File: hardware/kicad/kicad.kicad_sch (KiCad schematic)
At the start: 4 parts, among them U1 RP2040

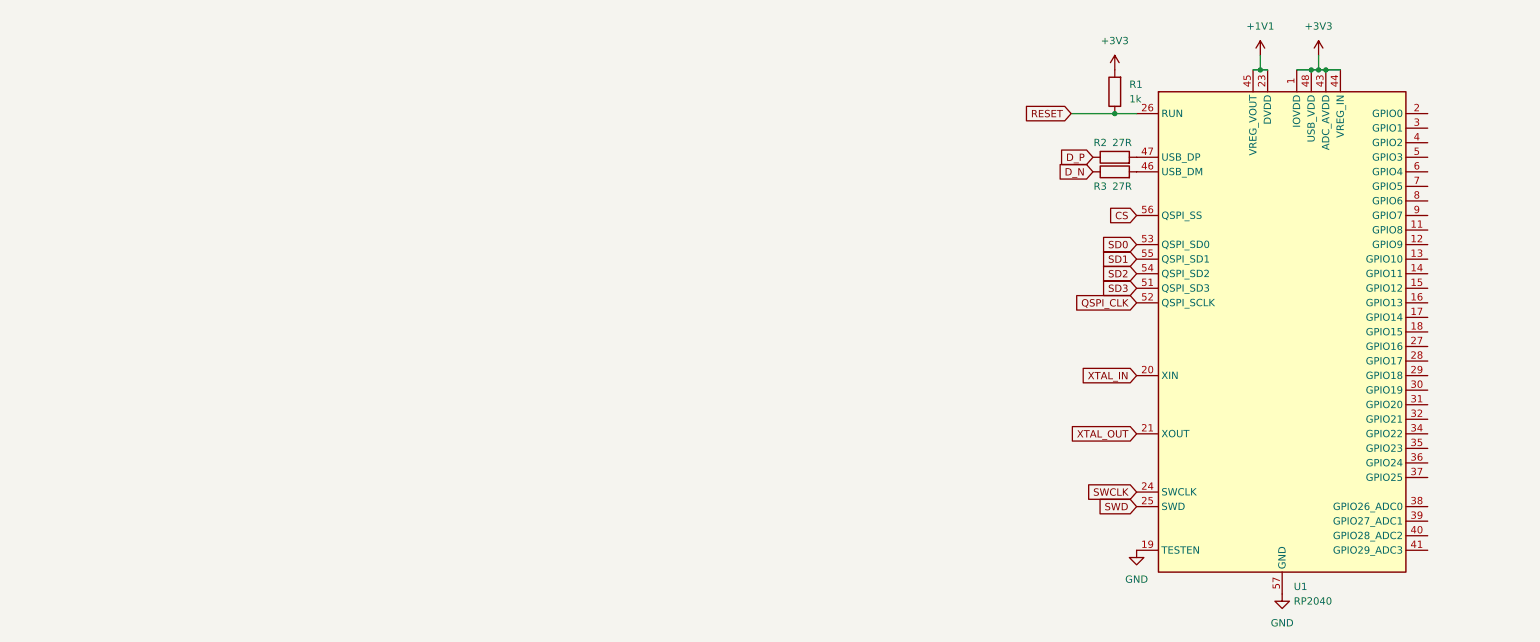
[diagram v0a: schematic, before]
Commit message: [30-8] update progress
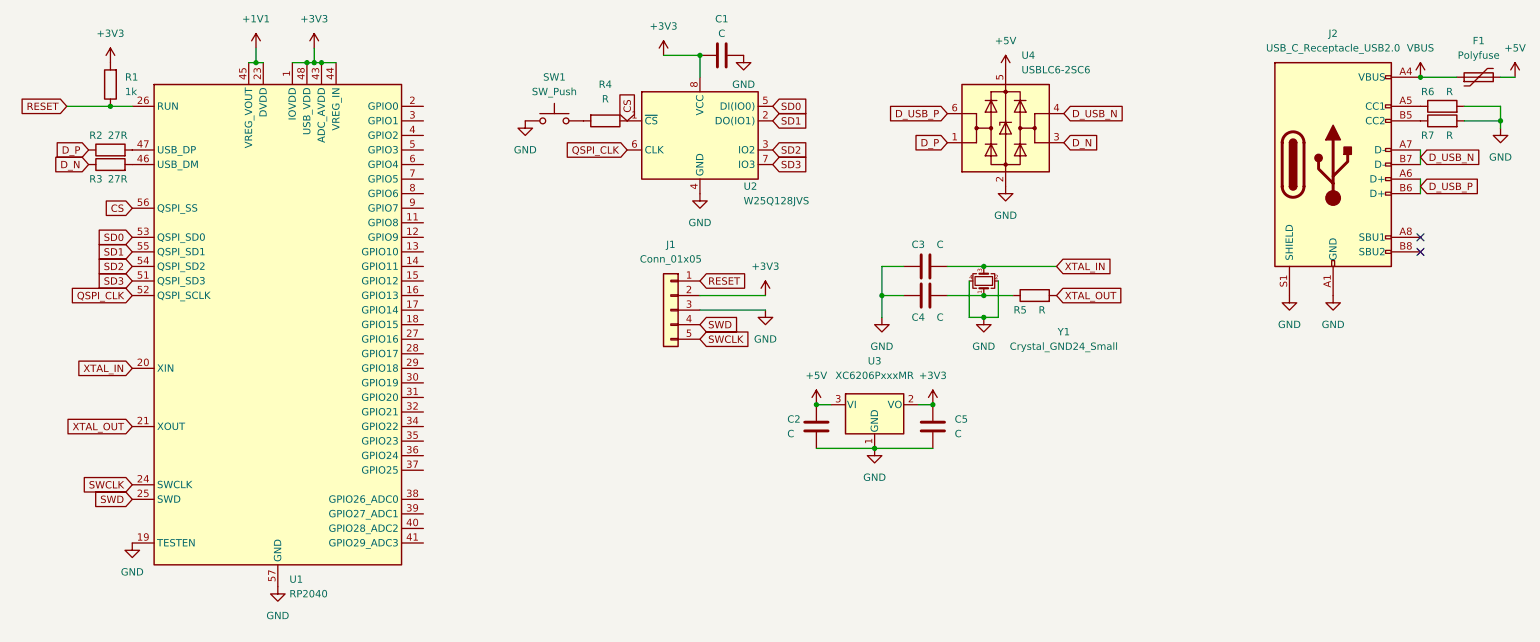
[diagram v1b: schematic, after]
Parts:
- added C1, C2, C3, C4, C5: C, Capacitor_SMD:C_0603_1608Metric_Pad1.08x0.95mm_HandSolder, symbol Device:C
- added F1: Polyfuse, Fuse:Fuse_0603_1608Metric_Pad1.05x0.95mm_HandSolder, symbol Device:Polyfuse
- added J1: Conn_01x05, Connector_PinHeader_2.54mm:PinHeader_1x05_P2.54mm_Vertical, symbol Connector_Generic:Conn_01x05
- added J2: USB_C_Receptacle_USB2.0, Connector_USB:USB_C_Receptacle_HRO_TYPE-C-31-M-12, symbol Connector:USB_C_Receptacle_USB2.0
- added R4, R5, R6, R7: R, Resistor_SMD:R_0603_1608Metric_Pad0.98x0.95mm_HandSolder, symbol Device:R
- added SW1: SW_Push, Button_Switch_SMD:SW_SPST_TL3342, symbol Switch:SW_Push
- added U2: W25Q128JVS, Package_SO:SOIC-8_5.23x5.23mm_P1.27mm, symbol Memory_Flash:W25Q128JVS
- added U3: XC6206PxxxMR, Package_TO_SOT_SMD:SOT-23, symbol Regulator_Linear:XC6206PxxxMR
- added U4: USBLC6-2SC6, Package_TO_SOT_SMD:SOT-23-6, symbol Power_Protection:USBLC6-2SC6
- added Y1: Crystal_GND24_Small, Crystal:Crystal_SMD_3225-4Pin_3.2x2.5mm_HandSoldering, symbol Device:Crystal_GND24_Small
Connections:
- net +3V3: now also C1.2, C5.1, J1.2 (Pin_2), U2.8 (VCC), U3.2 (VO)
- net CS: now also R4.1, U2.1 (~{CS})
- net D_N: now also U4.3 (I/O2)
- net D_P: now also U4.1 (I/O1)
- net GND: now also C1.1, C2.2, C3.1, C4.1, C5.2, J1.3 (Pin_3), J2.A1 (GND), J2.A12 (GND), J2.B1 (GND), J2.B12 (GND), J2.S1 (SHIELD), R6.2, R7.2, SW1.1, U2.4 (GND), U3.1 (GND), U4.2 (GND), Y1.2, Y1.4
- net QSPI_CLK: now also U2.6 (CLK)
- net RESET: now also J1.1 (Pin_1)
- net SD0: now also U2.5 (DI(IO0))
- net SD1: now also U2.2 (DO(IO1))
- net SD2: now also U2.3 (IO2)
- net SD3: now also U2.7 (IO3)
- net SWCLK: now also J1.5 (Pin_5)
- net SWD: now also J1.4 (Pin_4)
- net XTAL_IN: now also C3.2, Y1.3
- net XTAL_OUT: now also R5.2
- new net: R4.2, SW1.2
- new net: C4.2, R5.1, Y1.1
- new net: J2.A5 (CC1), R6.1
- new net: J2.B5 (CC2), R7.1
- new net +5V: C2.1, F1.2, U3.3 (VI), U4.5 (VBUS)
- new net D_USB_N: J2.A7 (D-), J2.B7 (D-), U4.4 (I/O2)
- new net D_USB_P: J2.A6 (D+), J2.B6 (D+), U4.6 (I/O1)
- new net VBUS: F1.1, J2.A4 (VBUS), J2.A9 (VBUS), J2.B4 (VBUS), J2.B9 (VBUS)
- no-connect marks 0 -> 2
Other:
- moved on the sheet: R1, R2, R3, U1

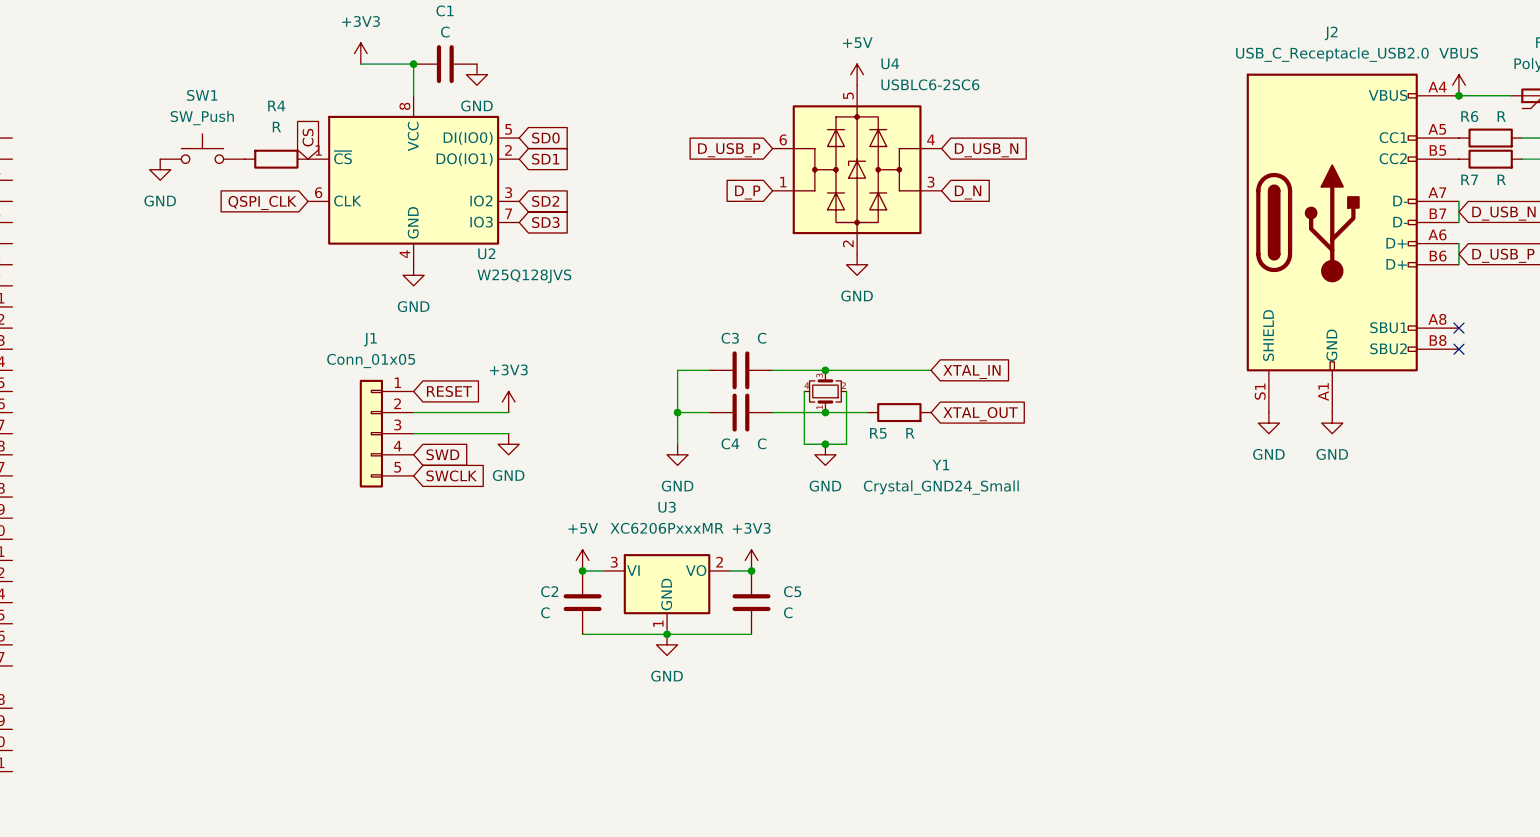
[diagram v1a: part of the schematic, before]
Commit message: [1-9] update progress
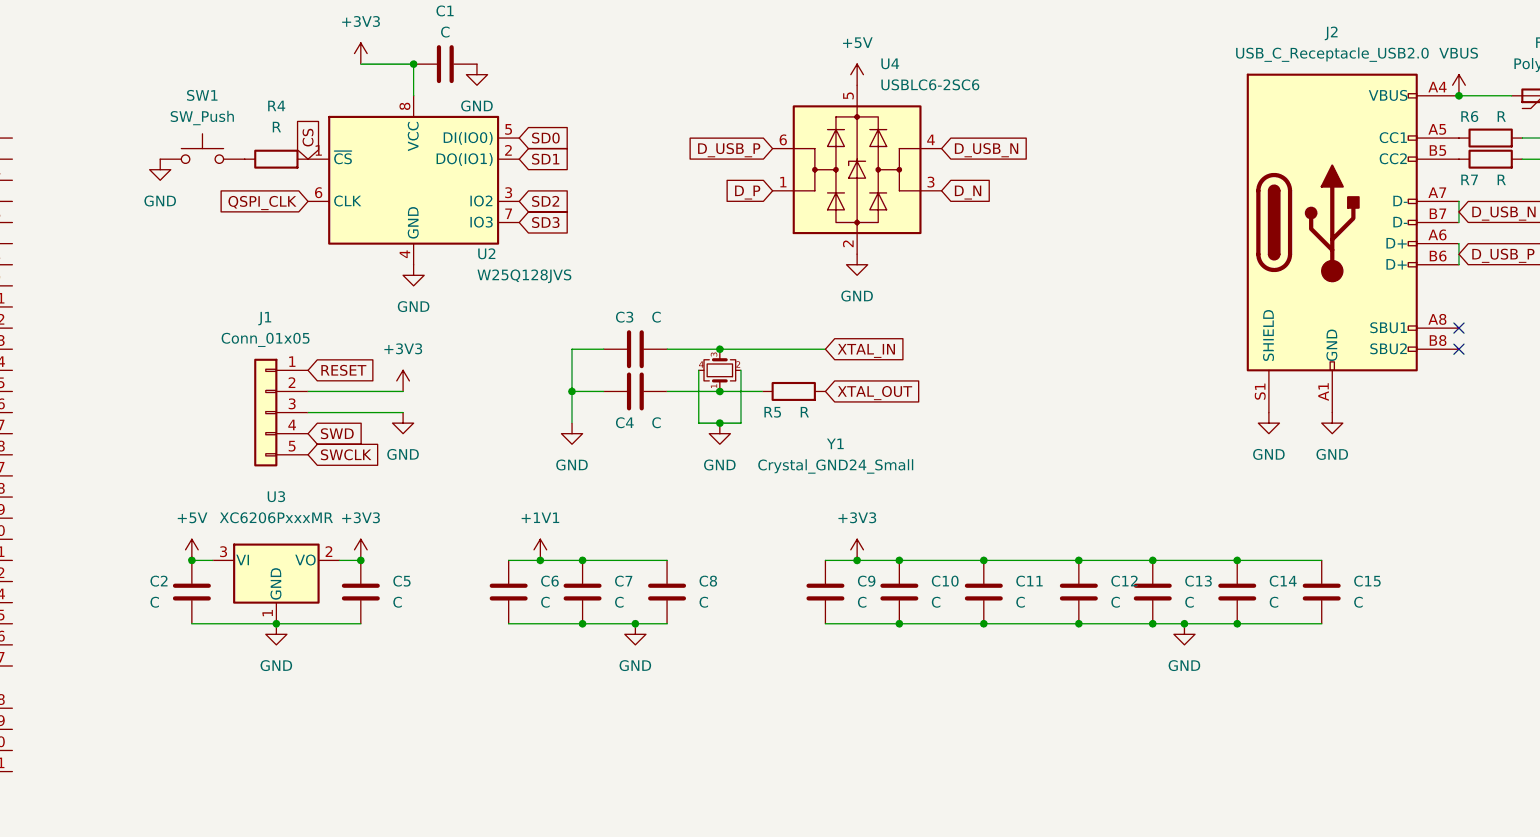
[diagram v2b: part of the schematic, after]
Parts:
- added C10, C11, C12, C13, C14, C15, C6, C7, C8, C9: C, Capacitor_SMD:C_0603_1608Metric_Pad1.08x0.95mm_HandSolder, symbol Device:C
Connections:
- net +1V1: now also C6.1, C7.1, C8.1
- net +3V3: now also C10.1, C11.1, C12.1, C13.1, C14.1, C15.1, C9.1
- net CS: now also R4.2; no longer R4.1
- net GND: now also C10.2, C11.2, C12.2, C13.2, C14.2, C15.2, C6.2, C7.2, C8.2, C9.2
- net at SW1.2: now also R4.1; no longer R4.2
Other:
- moved on the sheet: C2, C3, C4, C5, J1, R4, R5, U3, Y1
